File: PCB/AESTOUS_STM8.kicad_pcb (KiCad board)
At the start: 2 copper layers, 23 parts, among them J1 Conn_01x04_Male, J2 Conn_01x04_Male, J3 USB_B_Micro, U1 STM8S003F3P

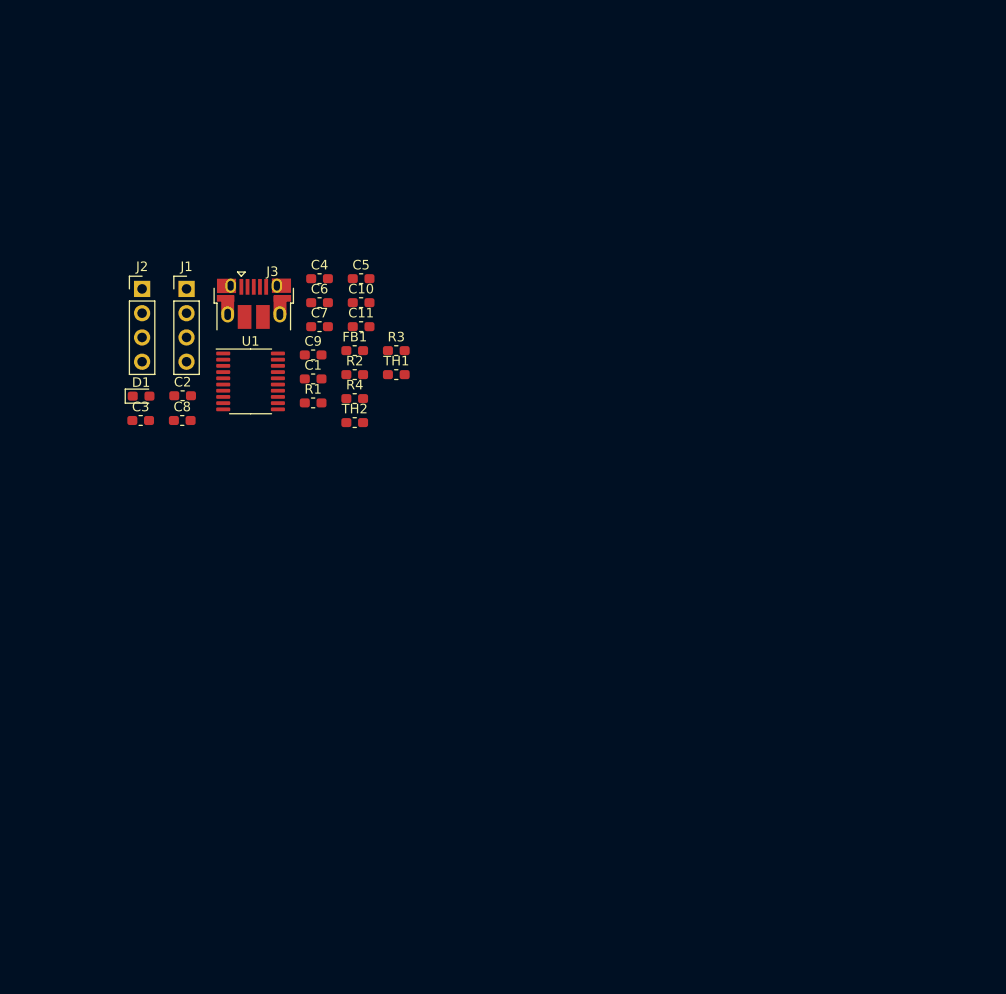
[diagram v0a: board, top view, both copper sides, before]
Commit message: new version
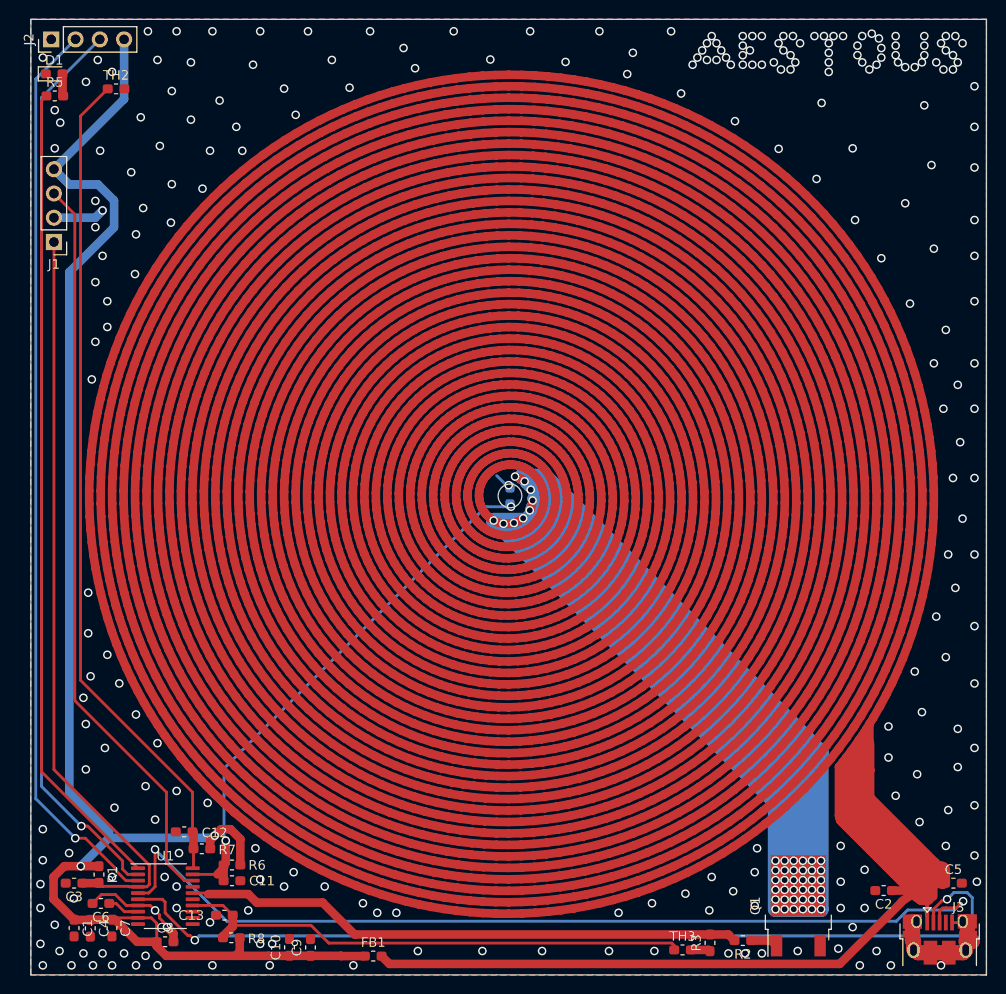
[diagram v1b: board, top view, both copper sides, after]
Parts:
- removed the C7 at (130.2, 82.2)
- removed R4: 0603WAF1002T5E, Resistor_SMD:R_0603_1608Metric_Pad1.05x0.95mm_HandSolder
- added C12: CL10A105KB8NNNC, Capacitor_SMD:C_0603_1608Metric_Pad1.05x0.95mm_HandSolder, F.Cu at (116.0, 135.0)
- added C13: CL10A105KB8NNNC, Capacitor_SMD:C_0603_1608Metric_Pad1.05x0.95mm_HandSolder, F.Cu at (120.2, 143.8)
- added C5: CL10A105KB8NNNC, Capacitor_SMD:C_0603_1608Metric_Pad1.05x0.95mm_HandSolder, F.Cu at (196.5, 140.4)
- added Q1: NCE2060K, Package_TO_SOT_SMD:TO-252-2, F.Cu at (180.3, 142.8)
- added R2: 0603WAF2700T5E, Resistor_SMD:R_0603_1608Metric_Pad1.05x0.95mm_HandSolder, F.Cu at (174.5, 146.4)
- added R6: 0603WAF1002T5E, Resistor_SMD:R_0603_1608Metric_Pad1.05x0.95mm_HandSolder, F.Cu at (121.0, 138.5)
- added R7: 0603WAF1002T5E, Resistor_SMD:R_0603_1608Metric_Pad1.05x0.95mm_HandSolder, F.Cu at (117.9, 136.8)
- added R8: 0603WAF1002T5E, Resistor_SMD:R_0603_1608Metric_Pad1.05x0.95mm_HandSolder, F.Cu at (121.0, 146.1)
- added TH3: NCP15XH103F03RC, Resistor_SMD:R_0603_1608Metric_Pad1.05x0.95mm_HandSolder, F.Cu at (168.2, 147.4)
- C1, C10, C11, C2, C3, C4, C6, C8, C9: value CL10B105KA8NNNC -> CL10A105KB8NNNC
- C7: renamed from C5; value 0603CG101J500NT -> CL10C101JB8NNNC
- J1, J2: value Conn_01x04_Male -> Conn_01x04
- R3: value 0603WAF1002T5E -> 0603WAF3002T5E
- TH1: moved to B.Cu
- moved J3 97.9 mm to (195.1, 146.3)
- moved C2 89.8 mm to (189.2, 141.2), turned to 180 degrees
- moved C7 72.8 mm to (108.5, 145.1), turned to 270 degrees
- moved C4 72.1 mm to (106.2, 145.1), turned to 270 degrees
- moved R3 70.1 mm to (171.1, 146.6), turned to 90 degrees
- moved C10 67.9 mm to (127.1, 147.1), turned to 90 degrees
- moved C6 66.9 mm to (107.3, 142.5), turned to 180 degrees
- moved FB1 63.4 mm to (135.8, 148.0)
- moved C1 62.7 mm to (104.5, 145.1), turned to 270 degrees
- moved C9 62.0 mm to (129.3, 147.1), turned to 90 degrees
- moved C11 59.5 mm to (121.0, 140.1)
- moved U1 54.6 mm to (114.1, 141.8)
- moved C8 54.6 mm to (114.0, 146.5)
- moved R1 54.2 mm to (107.1, 139.5), turned to 270 degrees
- moved C3 48.9 mm to (104.5, 140.4), turned to 180 degrees
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- renumbered R2 to R5
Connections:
- C1 pad 1: VDD -> +5VD
- C1 pad 2: GND -> 0
- C10 pad 1: +5V -> +5VD
- C10 pad 2: GND -> 0
- C11 pad 2: GND -> 0
- C2 pad 1: VDD -> Net-(Q1-Pad2)
- C2 pad 2: GND -> 0
- C3 pad 1: +5V -> /NRST
- C3 pad 2: GND -> 0
- C4 pad 1: +5V -> +5VD
- C4 pad 2: GND -> 0
- C6 pad 1: /NRST -> Net-(C6-Pad1)
- C6 pad 2: GND -> 0
- C7 pad 1: +5V -> +5VD
- C7 pad 2: GND -> 0
- C8 pad 1: +5V -> +5VD
- C8 pad 2: GND -> 0
- C9 pad 1: /ADC_IN4 -> +5VD
- C9 pad 2: GND -> 0
- D1 pad 1: GND -> 0
- FB1 pad 1: +5V -> +5VD
- J1 pad 1: +5V -> /NRST
- J1 pad 2: /UART_TX -> 0
- J1 pad 3: /UART_RX -> /SWIM
- J1 pad 4: GND -> +5VD
- J2 pad 1: +5V -> 0
- J2 pad 2: /SWIM -> /UART_RX
- J2 pad 3: GND -> /UART_TX
- J2 pad 4: /NRST -> +5VD
- J3 pad 1: VDD -> Net-(Q1-Pad2)
- J3 pad 5: GND -> 0
- J3 pad 6: GND -> 0
- R1 pad 1: +5V -> +5VD
- R3 pad 1: +5V -> 0
- R3 pad 2: /ADC_IN4 -> /TIM1_CH1
- TH1 pad 1: /ADC_IN4 -> /ADC_IN3
- TH1 pad 2: GND -> 0
- TH2 pad 1: /ADC_IN3 -> /ADC_IN4
- TH2 pad 2: GND -> 0
- U1 pad 7: GND -> 0
- U1 pad 8: Net-(C7-Pad1) -> Net-(C6-Pad1)
- U1 pad 9: +5V -> +5VD
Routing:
- net Net-(Q1-Pad2): track 0.00 -> 5653.8 mm, vias 0 -> 45
- net +5VD: track 0.00 -> 169.5 mm, vias 0 -> 2
- net /DM: track 0.00 -> 100.1 mm, vias 0 -> 2
- net /DP: track 0.00 -> 98.6 mm, vias 0 -> 2
- net /UART_RX: track 0.00 -> 95.7 mm, vias 0 -> 1
- net /UART_TX: track 0.00 -> 95.1 mm, vias 0 -> 1
- net /ADC_IN4: track 0.00 -> 87.7 mm
- net /LED: track 0.00 -> 85.2 mm
- net /NRST: track 0.00 -> 78.7 mm
- net /SWIM: track 0.00 -> 77.8 mm
- net /TIM1_CH1: track 0.00 -> 58.8 mm
- net /ADC_IN3: track 0.00 -> 58.0 mm, vias 0 -> 2
- net VDD: track 0.00 -> 57.4 mm
- net /ADC_IN2: track 0.00 -> 55.0 mm
- net 0: track 0.00 -> 35.3 mm, vias 0 -> 261
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- added copper zone on B.Cu, net 0
- added copper zone on F.Cu, net 0
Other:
- board outline added: 100 x 100 mm
- net class Default: clearance 0.2 -> 0.3; trace_width 0.25 -> 0.3; via_dia 0.8 -> 0.9; via_drill 0.4 -> 0.6
- rule trace_clearance: 0.2 -> 0.3
- rule trace_min: 0.2 -> 0.3
